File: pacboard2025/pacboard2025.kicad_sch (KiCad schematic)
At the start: 16 parts, among them U1 VL53L4CXV0DH/1, U10 D24V50F5, U11 Raspberry_PI_Zero_W, U12 Teensy_4.0, U2 VL53L4CXV0DH/1, U4 VL53L4CXV0DH/1, U5 VL53L4CXV0DH/1, U6 BNO085

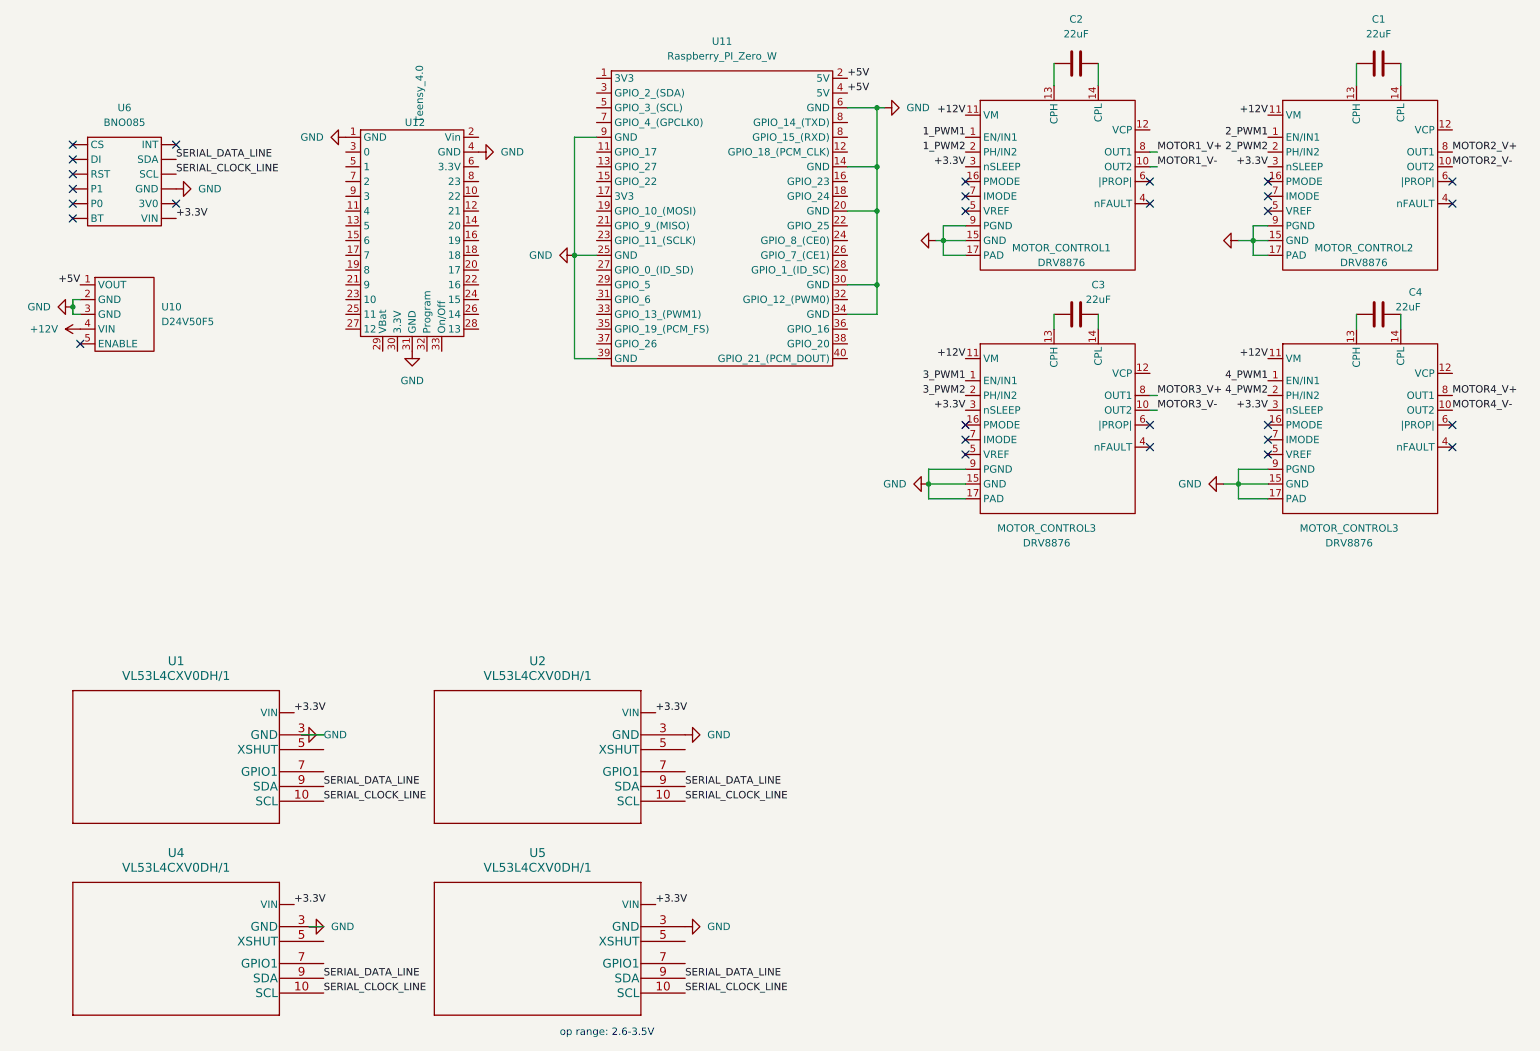
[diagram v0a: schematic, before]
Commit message: updated board design
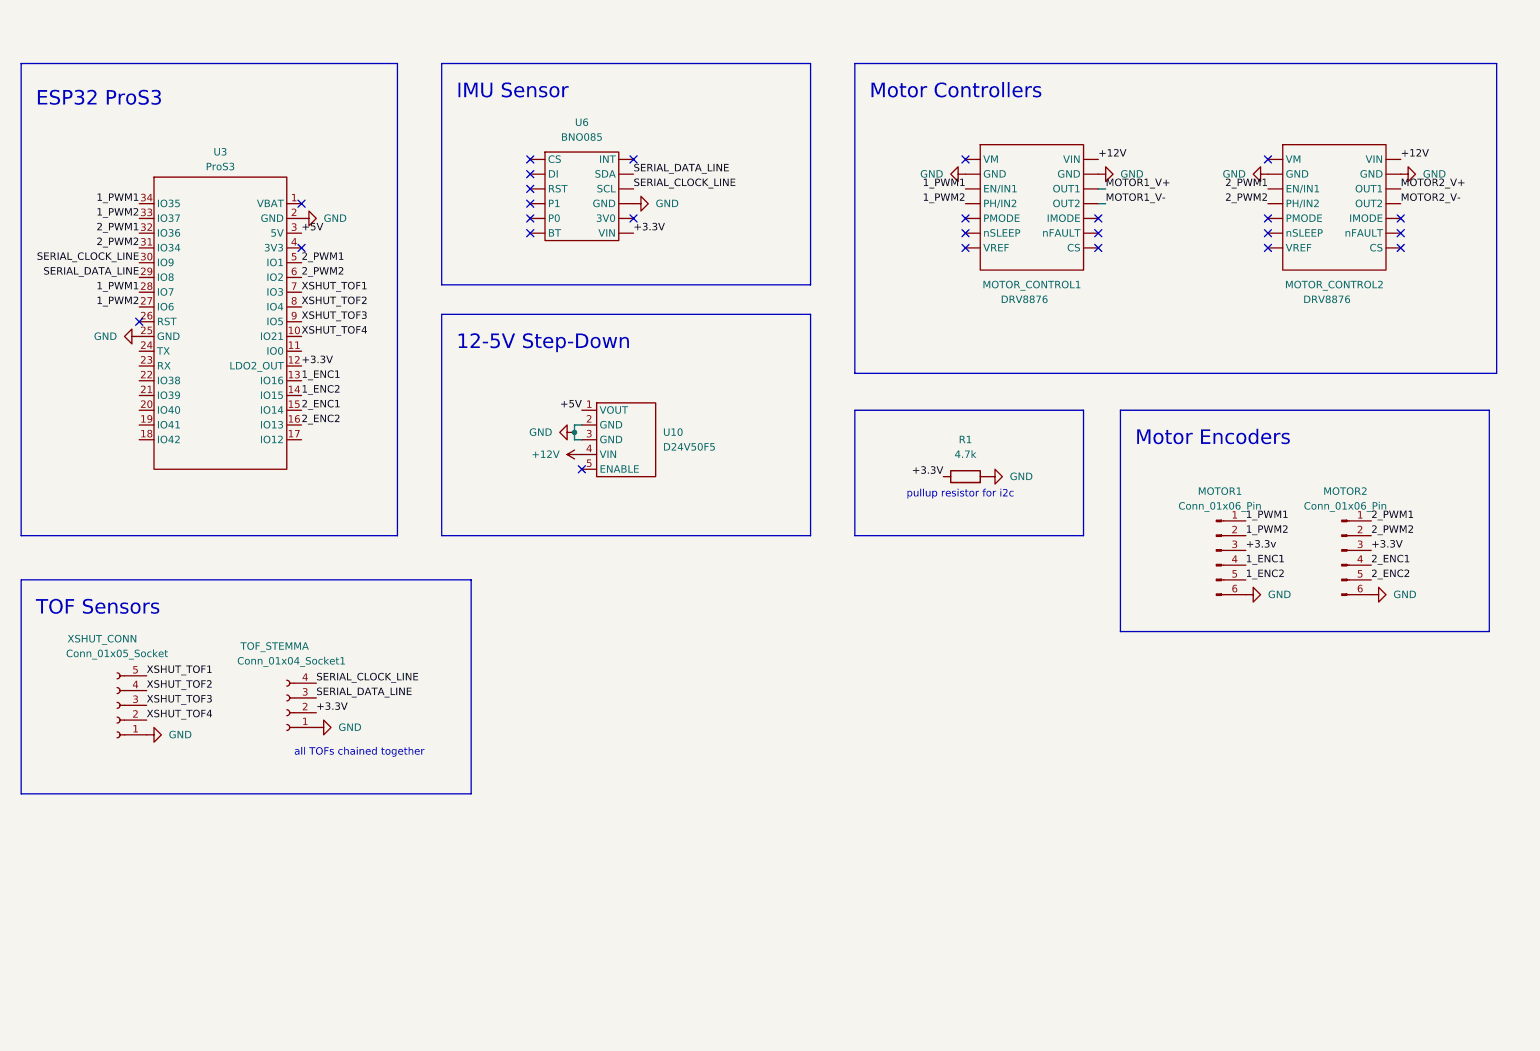
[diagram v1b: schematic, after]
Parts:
- removed C1, C2, C3, C4: 22uF, symbol Device:C
- removed MOTOR_CONTROL3 (x2): DRV8876, symbol board1_libs:DRV8876
- removed U1, U2, U4, U5: VL53L4CXV0DH/1, LGA12_STM, symbol board1_libs:VL53L4CXV0DH/1
- removed U11: Raspberry_PI_Zero_W, symbol board1_libs:Raspberry_PI_Zero_W
- removed U12: Teensy_4.0, symbol board1_libs:Teensy_4.0
- added Conn_01x04_Socket1: TOF_STEMMA, symbol Connector:Conn_01x04_Socket
- added MOTOR1, MOTOR2: Conn_01x06_Pin, symbol Connector:Conn_01x06_Pin
- added R1: 4.7k, symbol Device:R
- added U3: ProS3, symbol board1_libs:ProS3
- added XSHUT_CONN: Conn_01x05_Socket, symbol Connector:Conn_01x05_Socket
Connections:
- net +12V: now also MOTOR_CONTROL1. (nSLEEP), MOTOR_CONTROL2. (nSLEEP); no longer MOTOR_CONTROL1.11 (VM), MOTOR_CONTROL2.11 (VM)
- net +3.3V: now also Conn_01x04_Socket1.2 (Pin_2), MOTOR2.3 (Pin_3), R1.1, U3.12 (LDO2_OUT); no longer MOTOR_CONTROL1.3 (nSLEEP), MOTOR_CONTROL2.3 (nSLEEP)
- net +5V: now also U3.3 (5V)
- net 1_PWM1: now also MOTOR_CONTROL1. (nSLEEP), MOTOR1.1 (Pin_1), U3.28 (IO7), U3.34 (IO35); no longer MOTOR_CONTROL1.1 (EN/IN1)
- net 1_PWM2: now also MOTOR_CONTROL1. (nSLEEP), MOTOR1.2 (Pin_2), U3.27 (IO6), U3.33 (IO37); no longer MOTOR_CONTROL1.2 (PH/IN2)
- net 2_PWM1: now also MOTOR_CONTROL2. (nSLEEP), MOTOR2.1 (Pin_1), U3.32 (IO36), U3.5 (IO1); no longer MOTOR_CONTROL2.1 (EN/IN1)
- net 2_PWM2: now also MOTOR_CONTROL2. (nSLEEP), MOTOR2.2 (Pin_2), U3.31 (IO34), U3.6 (IO2); no longer MOTOR_CONTROL2.2 (PH/IN2)
- net GND: now also MOTOR_CONTROL1. (nSLEEP), MOTOR_CONTROL2. (nSLEEP), Conn_01x04_Socket1.1 (Pin_1), MOTOR1.6 (Pin_6), MOTOR2.6 (Pin_6), R1.2, U3.2 (GND), U3.25 (GND), XSHUT_CONN.1 (Pin_1); no longer MOTOR_CONTROL1.15 (GND), MOTOR_CONTROL1.17 (PAD), MOTOR_CONTROL1.9 (PGND), MOTOR_CONTROL2.15 (GND), MOTOR_CONTROL2.17 (PAD), MOTOR_CONTROL2.9 (PGND)
- net MOTOR1_V+: now also MOTOR_CONTROL1. (nSLEEP); no longer MOTOR_CONTROL1.8 (OUT1)
- net MOTOR1_V-: now also MOTOR_CONTROL1. (nSLEEP); no longer MOTOR_CONTROL1.10 (OUT2)
- net MOTOR2_V+: now also MOTOR_CONTROL2. (nSLEEP); no longer MOTOR_CONTROL2.8 (OUT1)
- net MOTOR2_V-: now also MOTOR_CONTROL2. (nSLEEP); no longer MOTOR_CONTROL2.10 (OUT2)
- net SERIAL_CLOCK_LINE: now also Conn_01x04_Socket1.4 (Pin_4), U3.30 (IO9)
- net SERIAL_DATA_LINE: now also Conn_01x04_Socket1.3 (Pin_3), U3.29 (IO8)
- new net +3.3v: MOTOR1.3 (Pin_3)
- new net 1_ENC1: MOTOR1.4 (Pin_4), U3.13 (IO16)
- new net 1_ENC2: MOTOR1.5 (Pin_5), U3.14 (IO15)
- new net 2_ENC1: MOTOR2.4 (Pin_4), U3.15 (IO14)
- new net 2_ENC2: MOTOR2.5 (Pin_5), U3.16 (IO13)
- new net XSHUT_TOF1: U3.7 (IO3), XSHUT_CONN.5 (Pin_5)
- new net XSHUT_TOF2: U3.8 (IO4), XSHUT_CONN.4 (Pin_4)
- new net XSHUT_TOF3: U3.9 (IO5), XSHUT_CONN.3 (Pin_3)
- new net XSHUT_TOF4: U3.10 (IO21), XSHUT_CONN.2 (Pin_2)
- no-connect marks 29 -> 26
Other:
- note added: "12-5V Step-Down"
- note added: "ESP32 ProS3"
- note added: "IMU Sensor"
- note added: "Motor Controllers"
- note added: "Motor Encoders"
- note added: "TOF Sensors"
- note added: "all TOFs chained together"
- note added: "pullup resistor for i2c"
- note removed: "op range: 2.6-3.5V"
- moved on the sheet: U10, U6
